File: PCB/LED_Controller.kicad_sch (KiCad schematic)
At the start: 44 parts, among them J1 Conn_01x04_Female, J2 Conn_01x06_Female, J3 Conn_01x06_Female, J4 Add. LED Strip, J5 Add. LED Strip, J7 Conn_01x02, Q1 MMBF170, Q10 BC817, Q2 MMBF170, Q3 MMBF170, Q4 MMBF170, Q9 BC817, SW1 SW_Push, SW2 SW_Push, U1 ESP32-WROOM-32, U2 NCP1117-5.0_SOT223, U3 NCP1117-3.3_SOT223

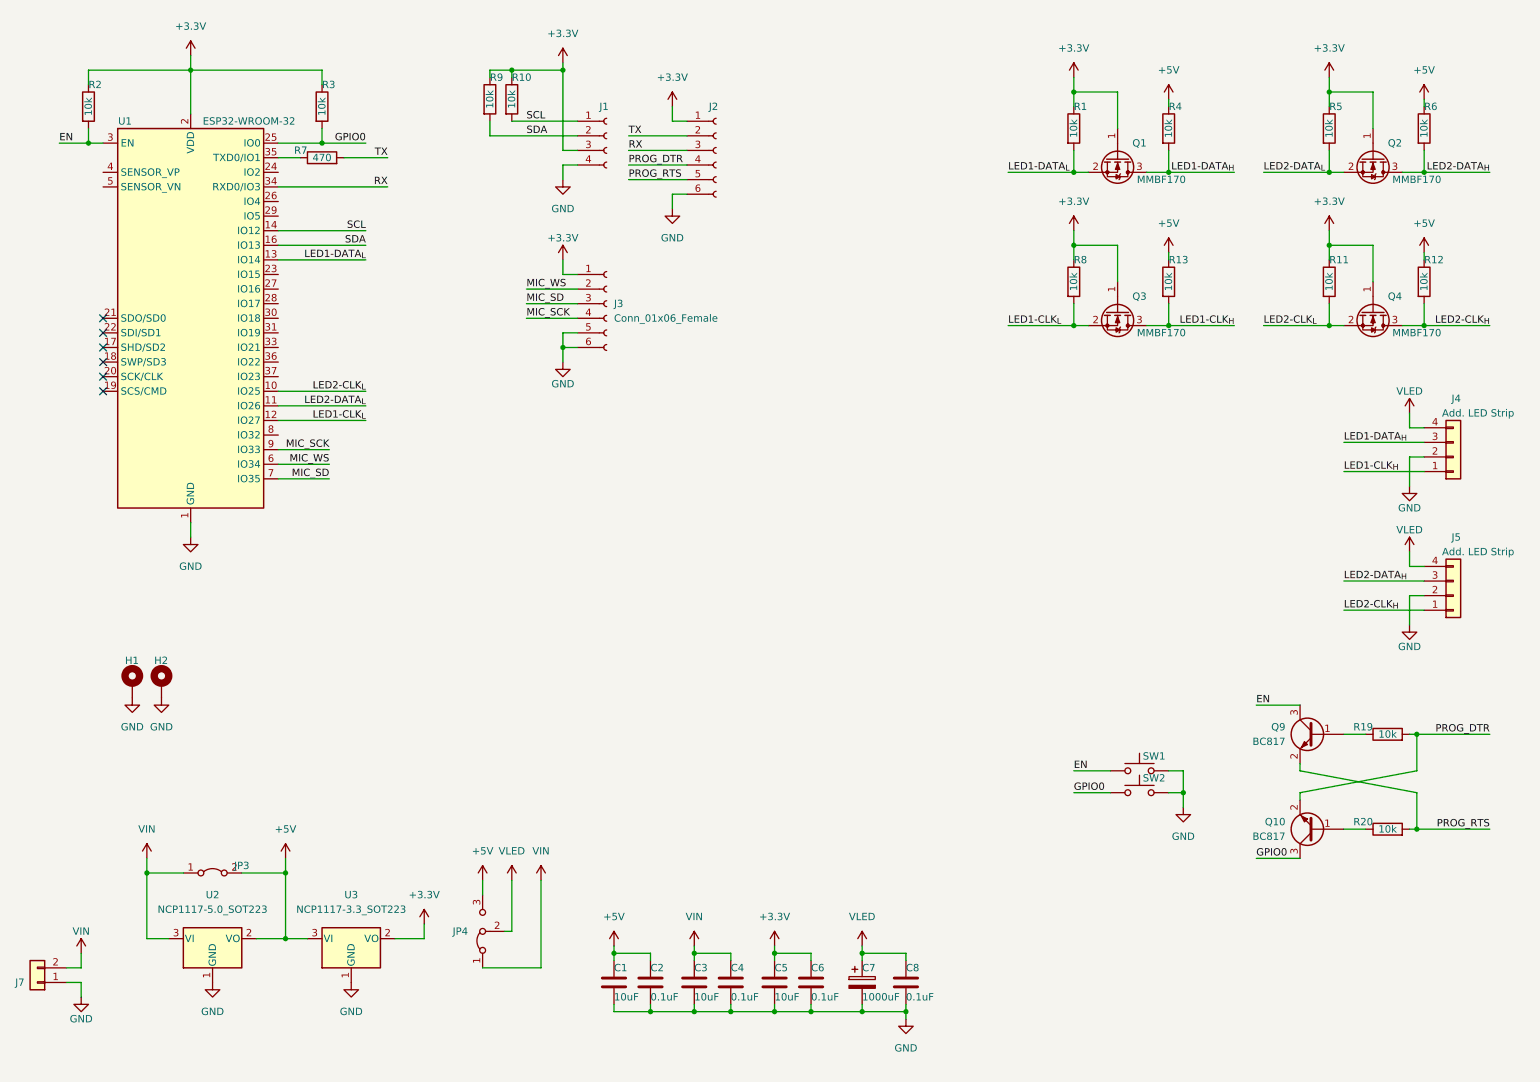
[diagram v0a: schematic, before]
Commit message: Rev 2.0 local push
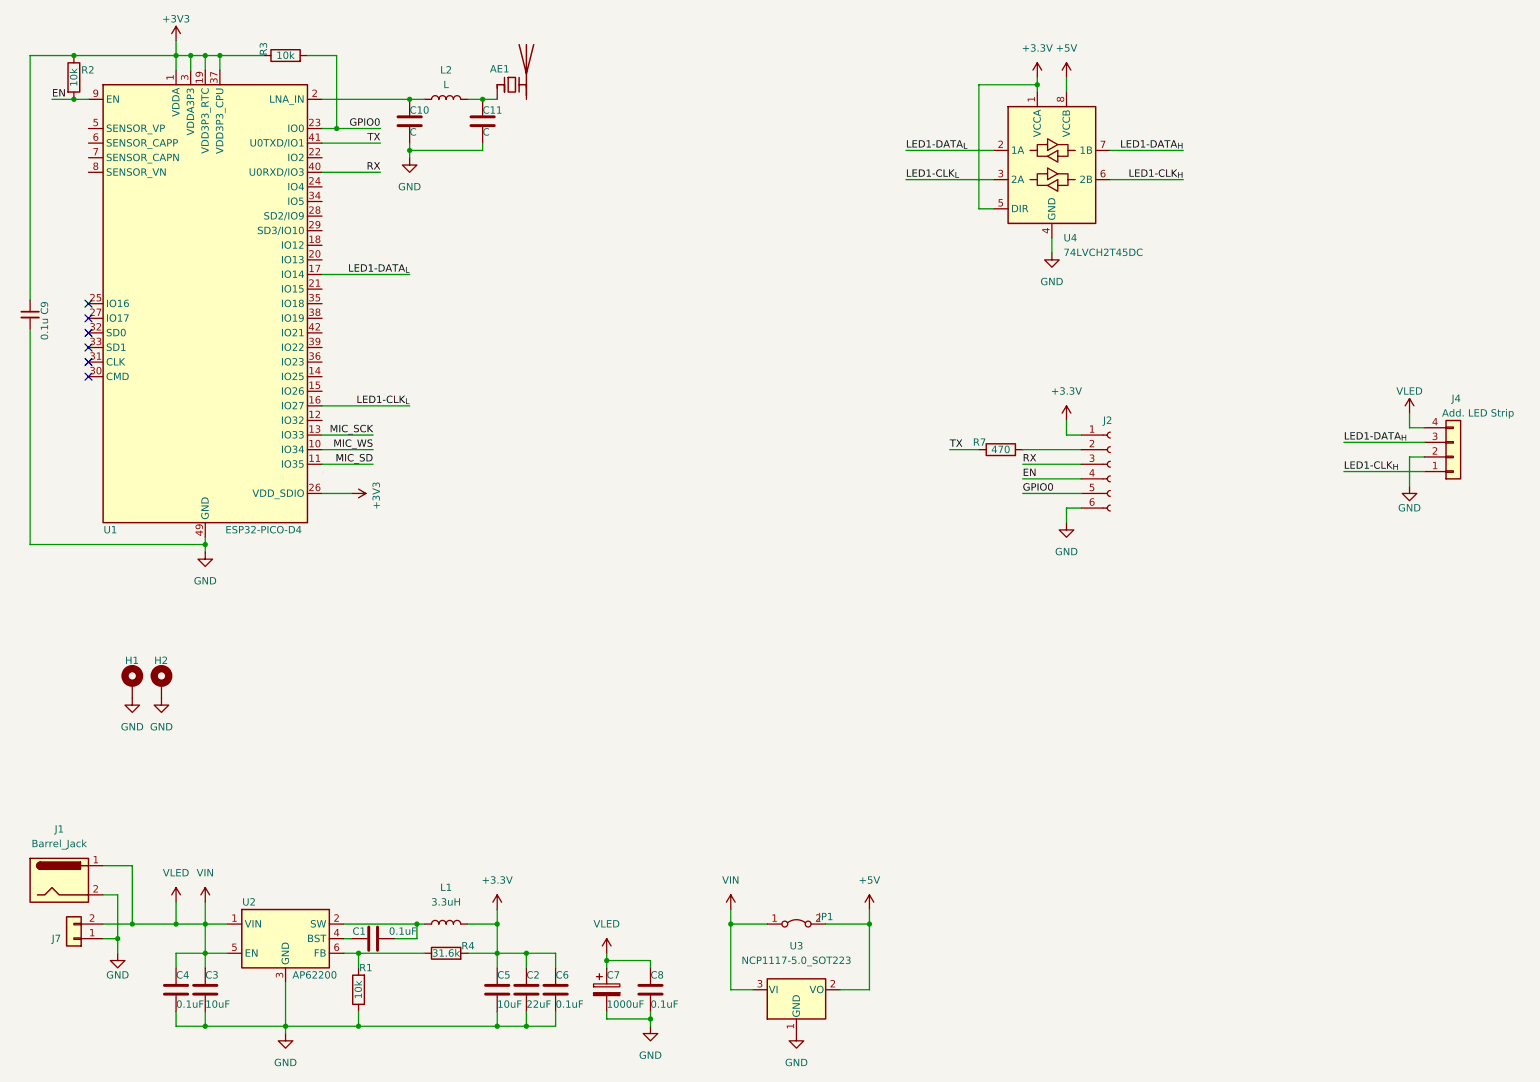
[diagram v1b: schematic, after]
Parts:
- removed J1: Conn_01x04_Female, Connector_PinHeader_2.54mm:PinHeader_2x02_P2.54mm_Vertical, symbol Connector:Conn_01x04_Female
- removed J3: Conn_01x06_Female, Connector_PinHeader_2.54mm:PinHeader_2x03_P2.54mm_Vertical, symbol Connector:Conn_01x06_Female
- removed J5: Add. LED Strip, TerminalBlock_Phoenix:TerminalBlock_Phoenix_MKDS-1,5-4-5.08_1x04_P5.08mm_Horizontal, symbol Connector_Generic:Conn_01x04
- removed JP3: Jumper_2_Bridged, Jumper:SolderJumper-2_P1.3mm_Bridged2Bar_Pad1.0x1.5mm, symbol Jumper:Jumper_2_Bridged
- removed JP4: Jumper_3_Bridged12, Jumper:SolderJumper-3_P1.3mm_Bridged2Bar12_Pad1.0x1.5mm, symbol Jumper:Jumper_3_Bridged12
- removed Q1, Q2, Q3, Q4: MMBF170, Package_TO_SOT_SMD:SOT-23, symbol Transistor_FET:MMBF170
- removed Q10, Q9: BC817, Package_TO_SOT_SMD:SOT-23, symbol Transistor_BJT:BC817
- removed R10, R11, R12, R13, R19, R20, R5, R6, R8, R9: 10k, Resistor_SMD:R_0805_2012Metric_Pad1.20x1.40mm_HandSolder, symbol Device:R
- removed SW1, SW2: SW_Push, Button_Switch_SMD:SW_Push_1P1T_NO_CK_KMR2, symbol Switch:SW_Push
- removed U1: ESP32-WROOM-32, RF_Module:ESP32-WROOM-32, symbol RF_Module:ESP32-WROOM-32
- removed U2: NCP1117-5.0_SOT223, Package_TO_SOT_SMD:SOT-223-3_TabPin2, symbol Regulator_Linear:NCP1117-5.0_SOT223
- removed U3: NCP1117-3.3_SOT223, Package_TO_SOT_SMD:SOT-223-3_TabPin2, symbol Regulator_Linear:NCP1117-3.3_SOT223
- added AE1: Antenna_Chip, RF_Antenna:Johanson_2450AT43F0100, symbol Device:Antenna_Chip
- added C10, C11: C, Capacitor_SMD:C_0805_2012Metric_Pad1.18x1.45mm_HandSolder, symbol Device:C
- added C9: 0.1u, Capacitor_SMD:C_0603_1608Metric, symbol Device:C_Small
- added J1: Barrel_Jack, Connector_BarrelJack:BarrelJack_Horizontal, symbol Connector:Barrel_Jack
- added JP1: Jumper_2_Bridged, Jumper:SolderJumper-2_P1.3mm_Bridged2Bar_Pad1.0x1.5mm, symbol Jumper:Jumper_2_Bridged
- added L1: 3.3uH, Inductor_SMD:L_1206_3216Metric_Pad1.22x1.90mm_HandSolder, symbol Device:L
- added L2: L, Inductor_SMD:L_0805_2012Metric_Pad1.05x1.20mm_HandSolder, symbol Device:L
- added U1: ESP32-PICO-D4, Package_DFN_QFN:QFN-48-1EP_7x7mm_P0.5mm_EP5.3x5.3mm, symbol RF_Module:ESP32-PICO-D4
- added U2: AP62200, Package_TO_SOT_SMD:SOT-563, symbol Regulator_Switching:AP62250Z6
- added U3: NCP1117-5.0_SOT223, Package_TO_SOT_SMD:SOT-223-3_TabPin2, symbol Regulator_Linear:NCP1117-5.0_SOT223
- added U4: 74LVCH2T45DC, Package_SO:VSSOP-8_2.3x2mm_P0.5mm, symbol Logic_LevelTranslator:74LVCH2T45DC
- C1: value 10uF -> 0.1uF
- C2: value 0.1uF -> 22uF; footprint Capacitor_SMD:C_0805_2012Metric_Pad1.18x1.45mm_HandSolder -> Capacitor_SMD:C_1206_3216Metric_Pad1.33x1.80mm_HandSolder
- C5: footprint Capacitor_SMD:C_0805_2012Metric_Pad1.18x1.45mm_HandSolder -> Capacitor_SMD:C_1206_3216Metric_Pad1.33x1.80mm_HandSolder
- R4: value 10k -> 31.6k
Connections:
- net PROG_DTR is gone; now on net EN: J2.4 (Pin_4)
- net PROG_RTS is gone; now on net GPIO0: J2.5 (Pin_5)
- net VLED is gone; now on net VIN: C7.1, C8.1, J4.4 (Pin_4)
- net +3V3: now also C2.1, R4.2, C9.1, L1.2, U1.1 (VDDA), U1.19 (VDD3P3_RTC), U1.26 (VDD_SDIO), U1.3 (VDDA3P3), U1.37 (VDD3P3_CPU), U1.4 (VDDA3P3), U1.43 (VDDA), U1.46 (VDDA), U4.1 (VCCA), U4.5 (DIR); no longer R1.1
- net +5V: now also JP1.2 (B), U3.2 (VO), U4.8 (VCCB); no longer C1.1, C2.1, R4.1
- net EN: now also U1.9 (EN)
- net GND: now also R1.1, C10.2, C11.2, C9.2, J1.2, U1.49 (GND), U2.3 (GND), U3.1 (GND), U4.4 (GND); no longer C1.2
- net GPIO0: now also U1.23 (IO0)
- net LED1-CLK_{H}: now also U4.6 (2B)
- net LED1-CLK_{L}: now also U1.16 (IO27), U4.3 (2A)
- net LED1-DATA_{H}: now also U4.7 (1B); no longer R4.2
- net LED1-DATA_{L}: now also U1.17 (IO14), U4.2 (1A); no longer R1.2
- net MIC_SCK: now also U1.13 (IO33)
- net MIC_SD: now also U1.11 (IO35)
- net MIC_WS: now also U1.10 (IO34)
- net RX: now also U1.40 (U0RXD/IO3)
- net TX: now also R7.1, U1.41 (U0TXD/IO1); no longer J2.2 (Pin_2), R7.2
- net VIN: now also J1.1, JP1.1 (A), U2.1 (VIN), U2.5 (EN), U3.3 (VI)
- new net: C1.2, L1.1, U2.2 (SW)
- new net: AE1.1 (FEED), C11.1, L2.2
- new net: J2.2 (Pin_2), R7.2
- new net: R1.2, R4.1, U2.6 (FB)
- new net: C10.1, L2.1, U1.2 (LNA_IN)
- new net: C1.1, U2.4 (BST)
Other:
- moved on the sheet: C3, C4, C5, C6, C7, C8, J2, J7, R7
